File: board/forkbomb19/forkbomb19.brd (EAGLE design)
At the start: 89.2 x 57 mm, 67 parts, among them T3 MMUN2133LT1G, U1 ESP-WROOM-03, U4 TPS61090RSAR, U5 MCP73871, X3 POT_GND, X4 POT_3V3, X5 POT_SIG

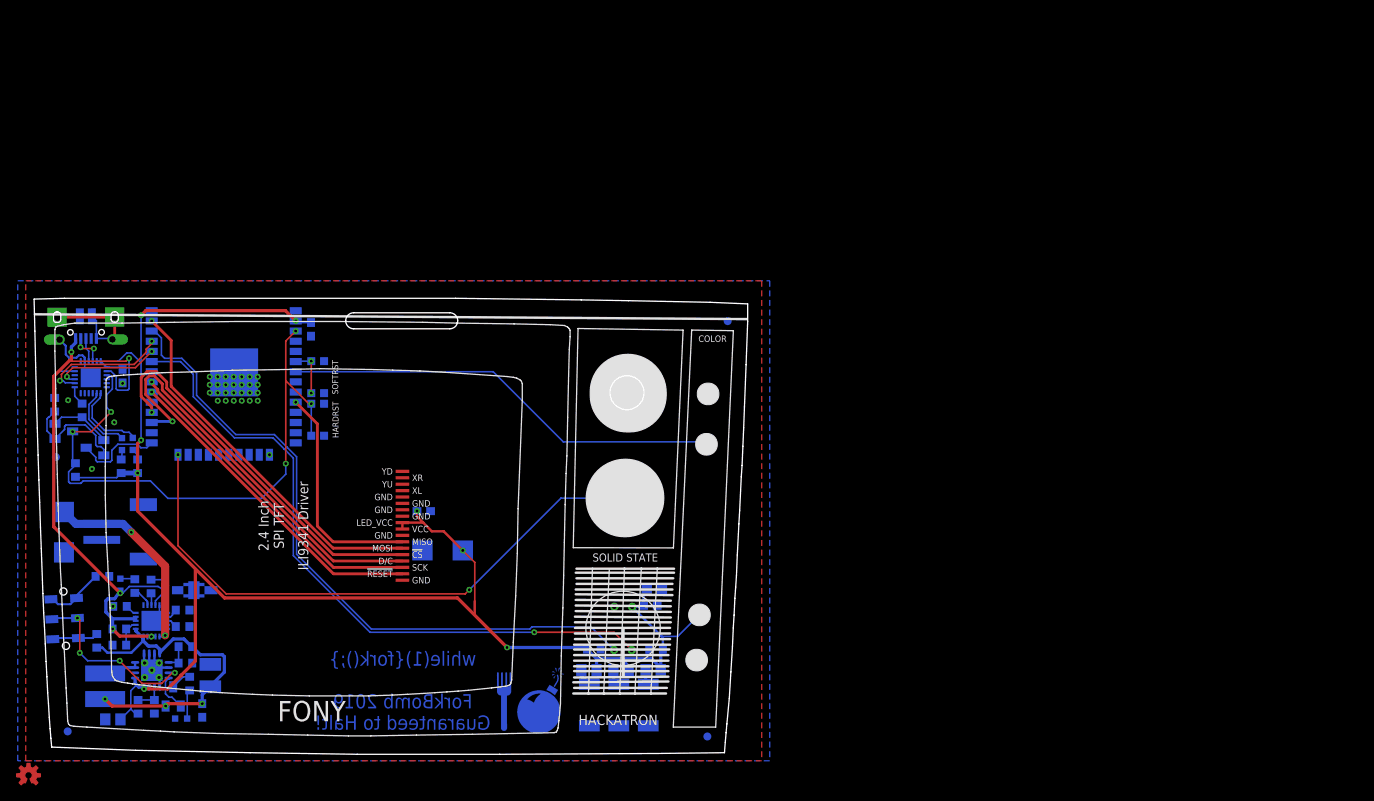
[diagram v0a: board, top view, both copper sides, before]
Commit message: performing board review
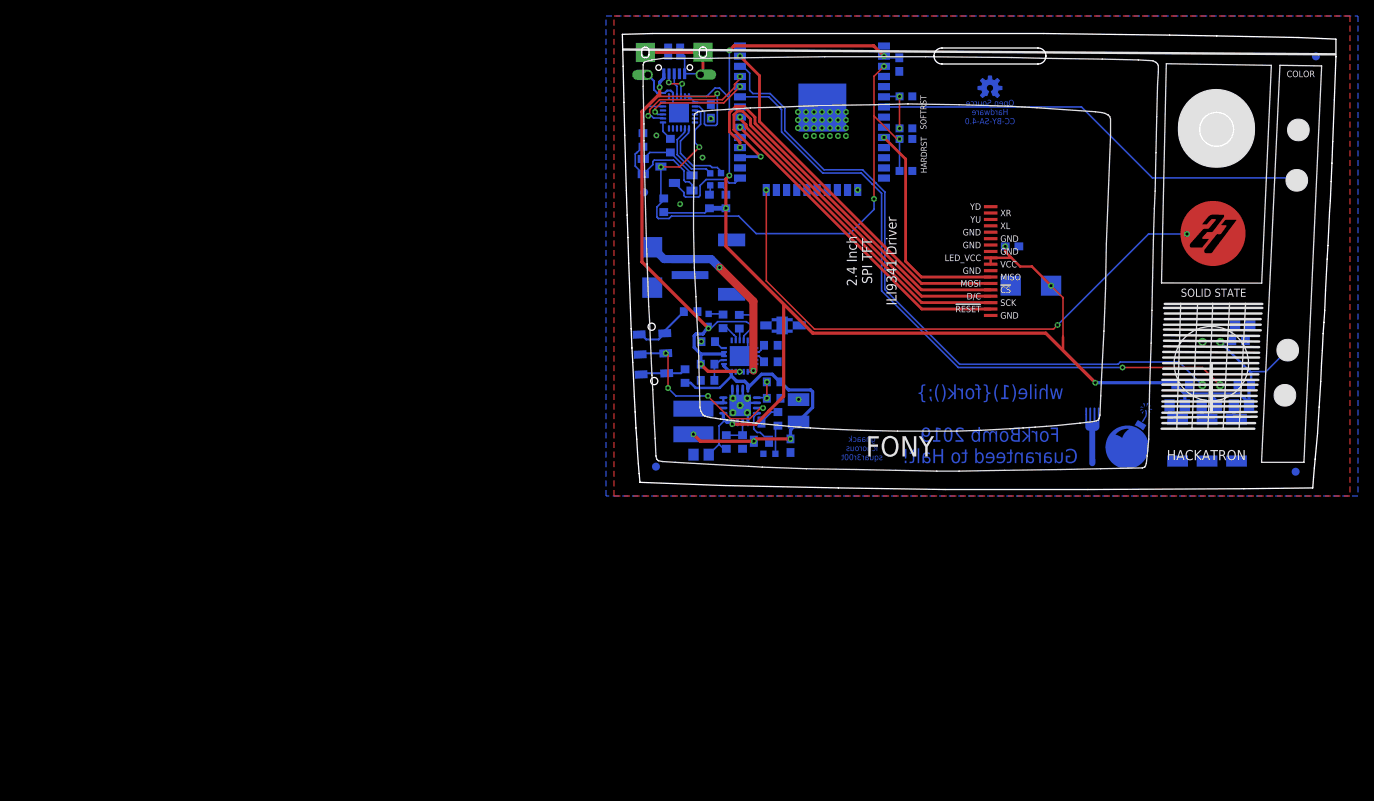
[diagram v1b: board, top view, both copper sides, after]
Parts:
- TOUCH: value TOUCHPAD -> TOUCHPADTOUCH_BLANK; device forkbomb19:TOUCHPAD_9.5MM -> forkbomb19:TOUCH_BLANK
- moved LOGO1 147.7 mm to (118.5, 83.1), flipped to the bottom
- moved X3 80.8 mm to (157.1, 77.9)
- moved X5 80.8 mm to (156.8, 71.6)
- moved C14 80.6 mm to (121.3, 63.3)
- moved C9 80.6 mm to (83.6, 80.2)
- moved CHRG 80.6 mm to (88.9, 54.1)
- moved FID1 80.6 mm to (76.8, 35.8)
- moved FID3 80.6 mm to (159.3, 87.0)
- moved FID4 80.6 mm to (75.3, 70.1)
- moved LOGO_G 80.6 mm to (145.7, 39.1)
- moved LOW_BATT 80.6 mm to (91.0, 37.4)
- moved R11 80.6 mm to (150.3, 46.0)
- moved R12 80.6 mm to (85.5, 68.9)
- moved R18 80.6 mm to (80.4, 47.1)
- moved R19 80.6 mm to (85.6, 38.8)
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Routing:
- net TOUCH2: track 74.7 -> 72.1 mm
- net GND: vias 33 -> 34
- net N$23: vias 0 -> 2
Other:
- outline, holes or cut-outs redrawn
- board text added: "Grant Haack"
- board text added: "Open Source Hardware CC-BY-SA-4.0"
- board text added: "ghaack ichorous squar3r00t"
